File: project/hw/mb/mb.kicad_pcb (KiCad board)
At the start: 2 copper layers, 80 x 50 mm, 18 parts, among them P1 CONN_02X04, P2 CONN_01X05, P3 CONN_01X05, SW1 SW_PUSH, SW2 SW_PUSH, U1 LPC1114/302

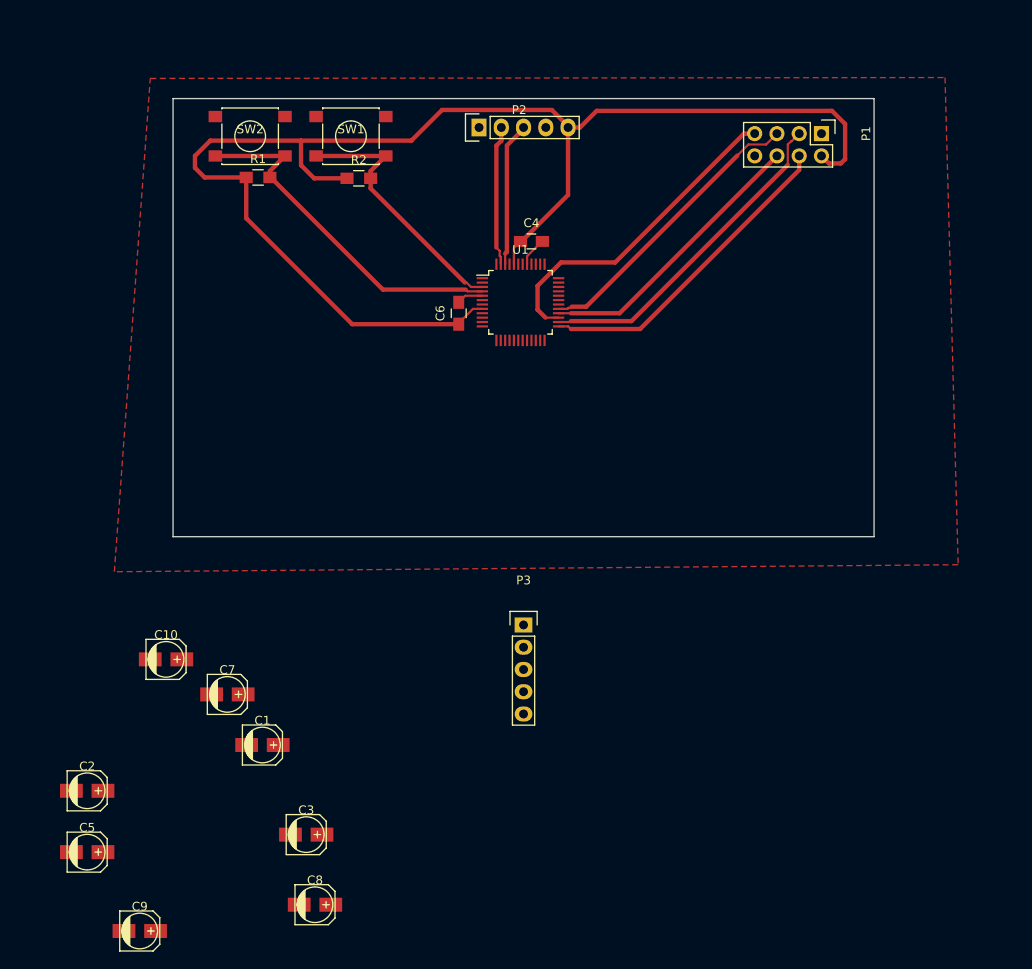
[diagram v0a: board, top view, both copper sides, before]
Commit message: motherboard design done
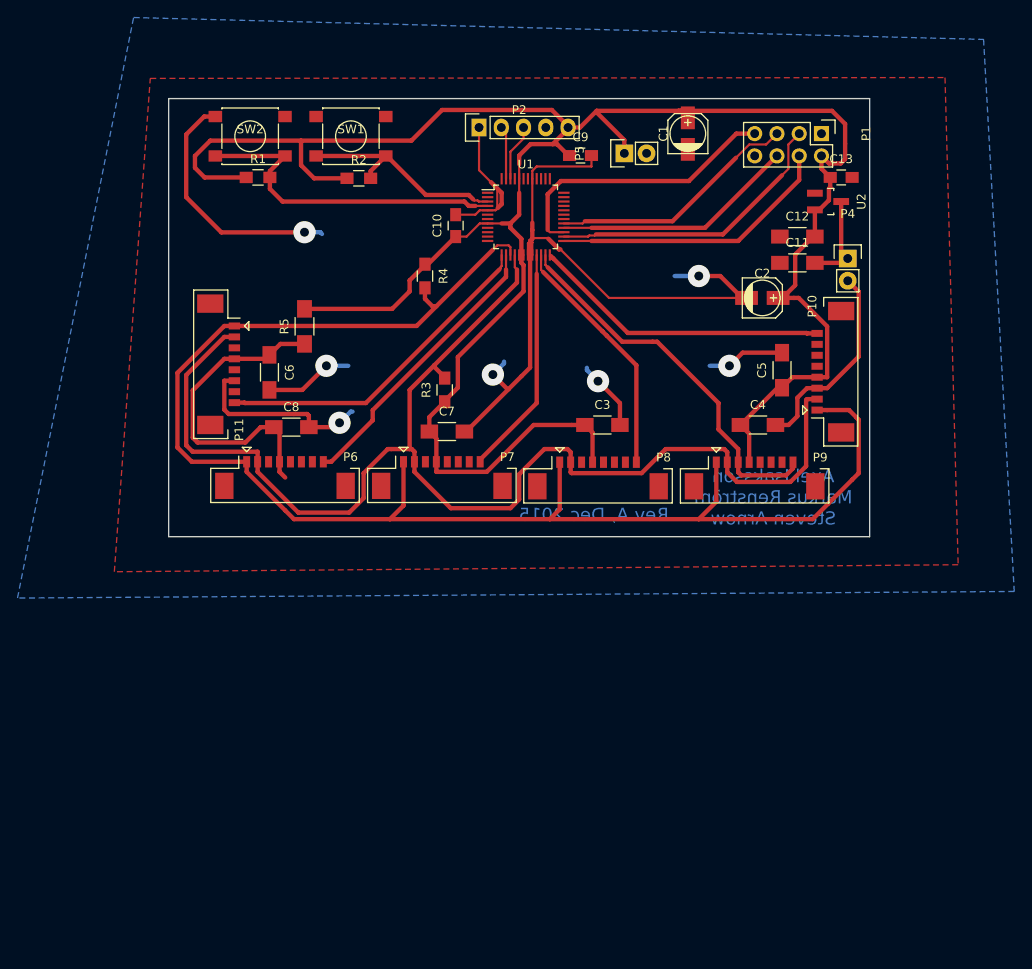
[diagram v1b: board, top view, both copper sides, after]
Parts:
- removed P3: CONN_01X05, Pin_Headers:Pin_Header_Straight_1x05
- added C11: 1u, Capacitors_SMD:C_1206_HandSoldering, F.Cu at (191.2, 68.8)
- added C12: 1u, Capacitors_SMD:C_1206_HandSoldering, F.Cu at (191.2, 65.8)
- added C13: 100n, Capacitors_SMD:C_0805_HandSoldering, F.Cu at (196.2, 59.0)
- added P10: CONN_01X08, Connectors_Molex:Connector_Molex_PicoBlade_53398-0871, F.Cu at (196.2, 81.2)
- added P11: CONN_01X08, Connectors_Molex:Connector_Molex_PicoBlade_53398-0871, F.Cu at (124.2, 80.3)
- added P4: CONN_01X02, Pin_Headers:Pin_Header_Straight_1x02, F.Cu at (197.0, 68.2)
- added P5: CONN_01X02, Pin_Headers:Pin_Header_Straight_1x02, F.Cu at (171.5, 56.2)
- added P6: CONN_01X08, Connectors_Molex:Connector_Molex_PicoBlade_53398-0871, F.Cu at (132.8, 94.2)
- added P7: CONN_01X08, Connectors_Molex:Connector_Molex_PicoBlade_53398-0871, F.Cu at (150.7, 94.2)
- added P8: CONN_01X08, Connectors_Molex:Connector_Molex_PicoBlade_53398-0871, F.Cu at (168.5, 94.2)
- added P9: CONN_01X08, Connectors_Molex:Connector_Molex_PicoBlade_53398-0871, F.Cu at (186.4, 94.2)
- added R3: 4k7, Resistors_SMD:R_0805_HandSoldering, F.Cu at (151.0, 83.2)
- added R4: 4k7, Resistors_SMD:R_0805_HandSoldering, F.Cu at (148.8, 70.2)
- added R5: 0, Resistors_SMD:R_1206_HandSoldering, F.Cu at (135.0, 76.0)
- added U2: mcp1700, Housings_SOT-23_SOT-143_TSOT-6:SOT-23_Handsoldering, F.Cu at (194.8, 61.8)
- C10, C9: value CP -> 100n; footprint Capacitors_SMD:c_elec_4x5.7 -> Capacitors_SMD:C_0805_HandSoldering
- C3, C5, C7, C8: value CP -> 1u; footprint Capacitors_SMD:c_elec_4x5.7 -> Capacitors_SMD:C_1206_HandSoldering
- C4, C6: value C -> 1u; footprint Capacitors_SMD:C_0805_HandSoldering -> Capacitors_SMD:C_1206_HandSoldering
- moved C9 101.8 mm to (166.5, 56.5)
- moved C5 96.5 mm to (189.5, 81.0), turned to 90 degrees
- moved C2 95.4 mm to (187.2, 72.8)
- moved C1 85.0 mm to (178.8, 54.0), turned to 90 degrees
- moved C10 59.5 mm to (152.2, 64.5), turned to 90 degrees
- moved C3 57.7 mm to (169.0, 87.2)
- moved C8 54.6 mm to (133.5, 87.5)
- moved C7 39.1 mm to (151.2, 88.0)
- moved C4 33.3 mm to (186.8, 87.2)
- moved C6 22.6 mm to (131.0, 81.2), turned to 270 degrees
- moved U1 9.77 mm to (160.2, 63.5)
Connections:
- U1 pad 13: (no net) -> /IMUA5
- U1 pad 14: (no net) -> /IMUA0
- U1 pad 17: (no net) -> +3V3
- U1 pad 18: (no net) -> +3V3
- U1 pad 19: (no net) -> GND
- U1 pad 20: (no net) -> GND
- U1 pad 21: (no net) -> /IMUA1
- U1 pad 22: (no net) -> /IMUA2
- U1 pad 23: (no net) -> /IMUA3
- U1 pad 24: (no net) -> /IMUA4
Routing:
- net GND: track 6.36 -> 209.7 mm, vias 0 -> 7
- net /SCL: track 0.00 -> 173.2 mm
- net /SDA: track 0.00 -> 149.3 mm
- net +3V3: track 157.9 -> 300.2 mm
- net /IMUA3: track 0.00 -> 43.7 mm
- net /IMUA5: track 0.00 -> 38.3 mm
- net /IMUA4: track 0.00 -> 34.6 mm
- net /IMUA0: track 0.00 -> 32.8 mm
- net /IMUA2: track 0.00 -> 28.2 mm
- net /IMUA1: track 0.00 -> 26.3 mm
- net Net-(C11-Pad2): track 0.00 -> 10.8 mm
- net /RX: track 16.5 -> 6.47 mm
- net /TX: track 16.0 -> 6.07 mm
- net /MISO: track 37.5 -> 32.5 mm
- net Net-(R2-Pad2): track 29.8 -> 25.0 mm
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- added copper zone on B.Cu, net GND
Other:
- net class Default: clearance 0.25 -> 0.24999
- rule trace_clearance: 0.25 -> 0.24999
- rule trace_min: 0.25 -> 0.009843
- rule via_min_size: 1.44 -> 0.056693
- board text added: "Axel Isaksson Markus Renström Steven Arnow"
- board text added: "Rev A, Dec 2015"
